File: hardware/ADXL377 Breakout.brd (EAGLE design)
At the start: 27.9 x 22.9 mm, 17 parts, among them U1 ADXL377

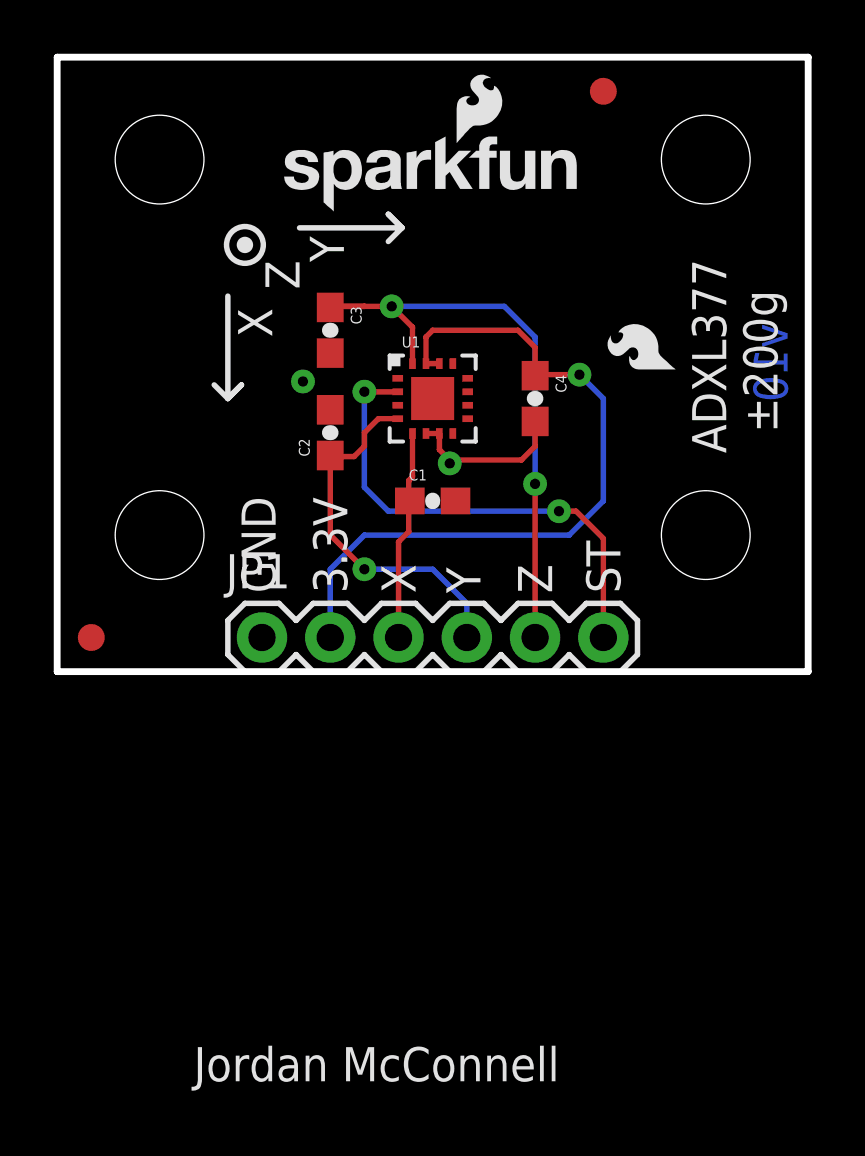
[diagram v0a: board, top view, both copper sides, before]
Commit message: v10, ready for reds
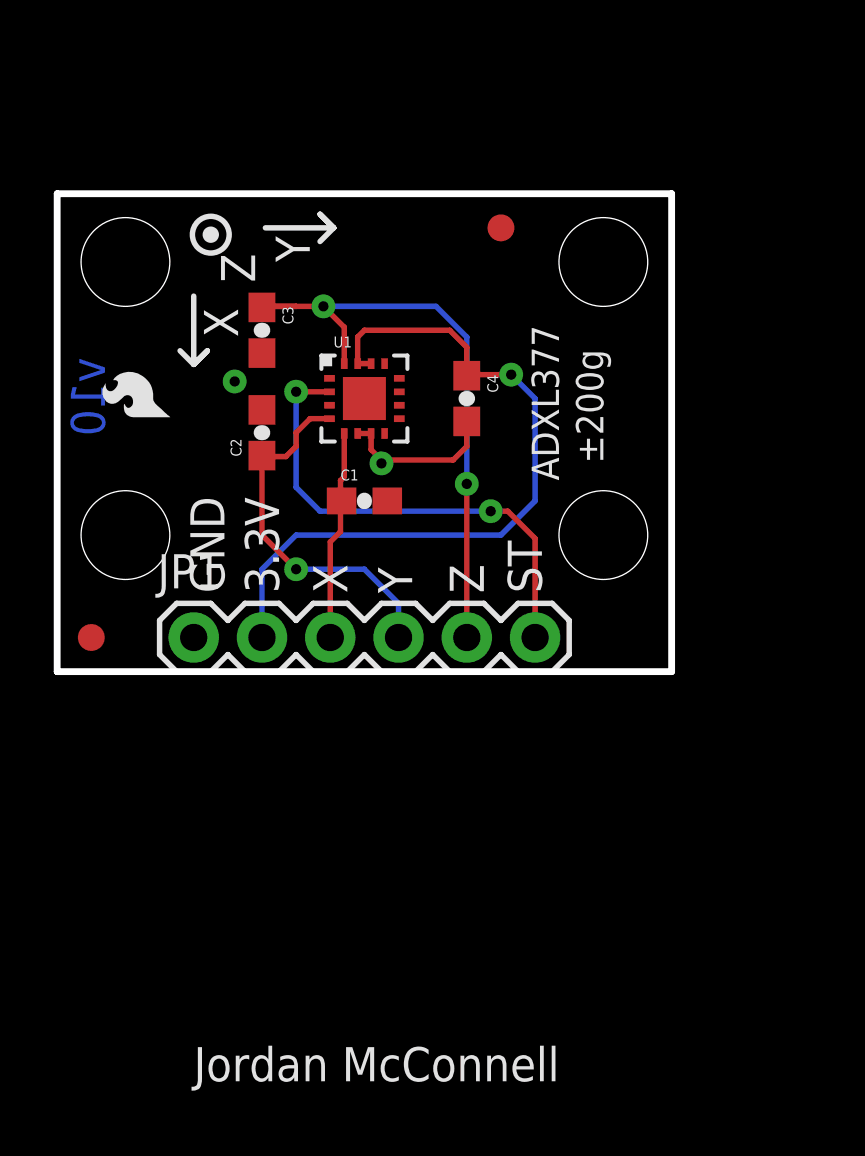
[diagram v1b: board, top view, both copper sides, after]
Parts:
- removed LOGO5: SFE_LOGO_NAME_FLAME.1_INCH, SparkFun-Aesthetics:SFE_LOGO_NAME_FLAME_.1
- moved LOGO1 18.9 mm to (4.57, 9.14)
- moved LOGO3 9.21 mm to (18.3, 15.1)
- moved FID1 6.35 mm to (16.5, 16.5)
- moved STANDOFF1 5.39 mm to (20.3, 15.2)
- moved STANDOFF3 4.02 mm to (2.54, 15.2)
- moved STANDOFF4 3.81 mm to (20.3, 5.08)
- moved LOGO2 2.84 mm to (20.3, 10.2)
- moved C1 2.54 mm to (11.4, 6.35)
- moved C4 2.54 mm to (15.2, 10.2)
- moved U1 2.54 mm to (11.4, 10.2)
- moved C2 2.54 mm to (7.62, 8.89)
- moved C3 2.54 mm to (7.62, 12.7)
- moved JP1 2.54 mm to (5.08, 1.27)
- moved STANDOFF2 1.27 mm to (2.54, 5.08)
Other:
- board size 27.9 x 22.9 mm -> 22.9 x 17.8 mm
